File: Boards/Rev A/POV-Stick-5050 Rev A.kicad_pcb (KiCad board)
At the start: 2 copper layers, 115.6 x 9.3 mm, 23 parts, among them J1 ISP_Header, J2 Batt Conn, SW1 Power Switch, U1 ATTINY85-20SU, U10 APA102C, U11 APA102C, U2 APA102C, U3 APA102C, U4 APA102C, U5 APA102C, U6 APA102C, U7 APA102C, U8 APA102C, U9 APA102C

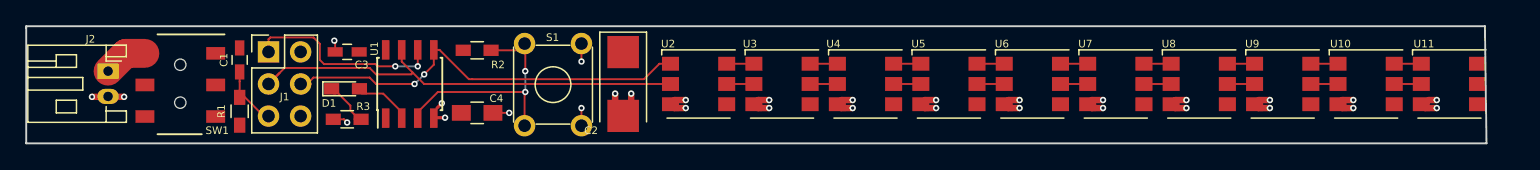
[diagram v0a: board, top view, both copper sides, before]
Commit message: Finished layout
Need to add Flamingo logo
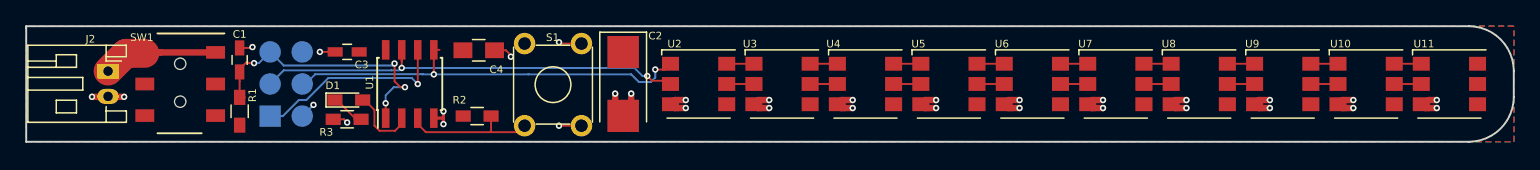
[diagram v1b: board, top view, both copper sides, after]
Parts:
- J1: footprint Pin_Headers:Pin_Header_Straight_2x03_Pitch2.54mm -> MyConnectors:ISP_Header_Pogo_2x03_Pitch2.54mm; moved to B.Cu
- moved R2 5.21 mm to (126.2, 57.1)
- moved J1 5.08 mm to (109.9, 57.1)
- moved C4 4.95 mm to (126.4, 51.9)
- moved D1 0.92 mm to (116.1, 55.9)
- moved SW1 0.08 mm to (105.5, 52.1)
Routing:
- net Net-(C1-Pad1): track 5.07 -> 22.1 mm, vias 0 -> 4
- net /PIN3/SW3: track 19.1 -> 12.0 mm, vias 2 -> 0
- net Net-(J2-Pad1): track 3.50 -> 9.10 mm
- net GND: track 41.4 -> 45.0 mm, vias 30 -> 32
- net Net-(D1-Pad2): track 4.26 -> 6.00 mm
- net +BATT: track 0.00 -> 1.26 mm, vias 0 -> 1
- net Net-(D1-Pad1): track 4.25 -> 3.41 mm
- net /SCK/WS2812Clock: track 36.4 -> 35.6 mm, vias 0 -> 2
- net /MOSI/WS2812Data: track 33.8 -> 33.1 mm
- net (no net): track 0.54 -> 0.00 mm, vias 1 -> 0
- net /PIN6/SCK: track 15.9 -> 16.3 mm, vias 2 -> 1
- added copper zone on F.Cu, net +BATT
- added copper zone on B.Cu, net GND
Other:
- board size 115.6 x 9.3 mm -> 117.7 x 9.1 mm
- board text added: "POV Stick 5050 Rev A Paul Blackburn 2018 GitHub: @individual61"
